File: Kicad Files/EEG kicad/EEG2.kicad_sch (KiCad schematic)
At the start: 273 parts, among them J1 Conn_02x20_Top_Bottom, J2 Conn_01x05_Pin, U1 INA823, U10 LF356M, U11 LF356M, U12 LF356M, U13 LF356M, U14 LF356M, U15 LF356M, U16 LF356M, U17 LF356M, U18 LF356M, U19 LF356M, U2 INA823, U20 LF356M, U21 LF356M, U22 LF356M, U23 LF356M, U24 LF356M, U25 LF356M, U26 AD5293, U27 AD5293, U28 AD5293, U29 AD5293, U3 INA823, U30 AD5293, U31 Teensy4.1, U32 AD5293, U33 AD5293, U34 AD5293, U35 AD5293, U36 AD5293, U37 LF356M, U38 LF356M, U39 LF356M, U4 INA823, U40 LF356M, U41 LF356M, U42 LF356M, U43 LF356M, U44 LF356M, U45 LF356M, U46 LF356M, U47 LF356M, U48 LF356M, U49 LF356M, U5 INA823, U50 LF356M, U51 LF356M, U52 LF356M, U53 LF356M, U54 LF356M, U55 LF356M, U56 LF356M, U57 INA823, U58 INA823, U59 INA823, U6 LF356M, U60 INA823, U61 INA823, U7 LF356M, U8 LF356M, U9 LF356M

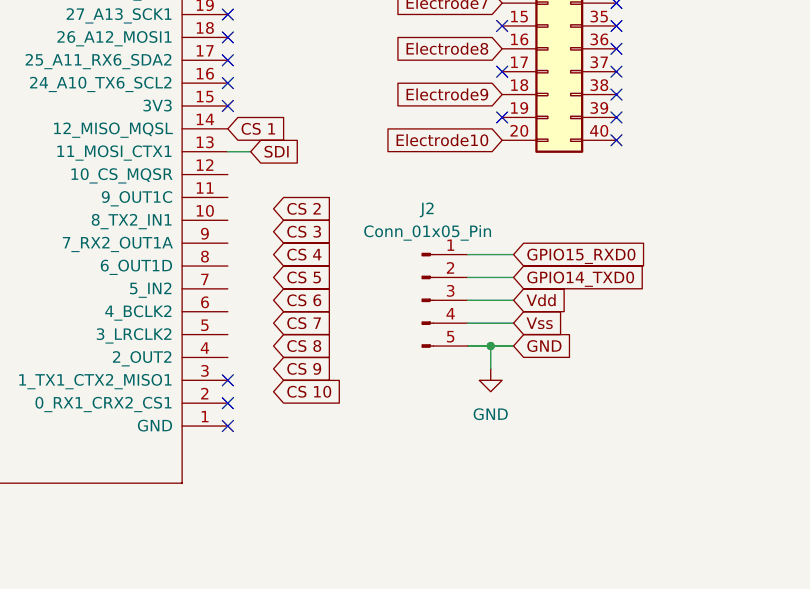
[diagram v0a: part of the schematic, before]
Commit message: AR & EEG corrected
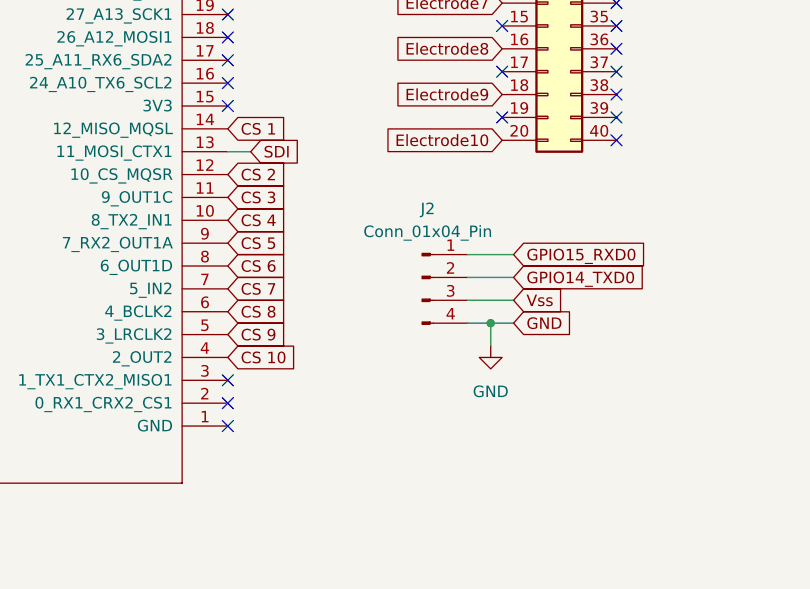
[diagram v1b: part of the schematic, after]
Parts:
- removed J2: Conn_01x05_Pin, Connector_PinHeader_1.27mm:PinHeader_1x05_P1.27mm_Vertical, symbol Connector:Conn_01x05_Pin
- added J2: Conn_01x04_Pin, Connector_PinHeader_1.27mm:PinHeader_1x04_P1.27mm_Vertical, symbol Connector:Conn_01x04_Pin
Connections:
- net CS 10: now also U31.4 (2_OUT2)
- net CS 2: now also U31.12 (10_CS_MQSR)
- net CS 3: now also U31.11 (9_OUT1C)
- net CS 4: now also U31.10 (8_TX2_IN1)
- net CS 5: now also U31.9 (7_RX2_OUT1A)
- net CS 6: now also U31.8 (6_OUT1D)
- net CS 7: now also U31.7 (5_IN2)
- net CS 8: now also U31.6 (4_BCLK2)
- net CS 9: now also U31.5 (3_LRCLK2)
- net GND: now also J2.4 (Pin_4)
- net GPIO14_TXD0: now also J2.2 (Pin_2)
- net GPIO15_RXD0: now also J2.1 (Pin_1)
- net Vss: now also J2.3 (Pin_3)
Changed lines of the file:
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@@
 	)
 	(junction
-		(at 321.31 92.71)
+		(at 321.31 90.17)
 		(diameter 0)
 		(color 0 0 0 0)
@@
 	(wire
 		(pts
-			(xy 321.31 92.71) (xy 321.31 95.25)
+			(xy 321.31 90.17) (xy 321.31 92.71)
 		)
 		(stroke
@@
 	(wire
 		(pts
-			(xy 318.77 87.63) (xy 323.85 87.63)
-		)
-		(stroke
-			(width 0)
-			(type default)
-		)
-	)
-	(wire
-		(pts
 			(xy 219.71 360.68) (xy 222.25 360.68)
 		)
@@
 	(wire
 		(pts
-			(xy 318.77 92.71) (xy 321.31 92.71)
-		)
-		(stroke
-			(width 0)
-			(type default)
-		)
-	)
-	(wire
-		(pts
-			(xy 318.77 90.17) (xy 323.85 90.17)
+			(xy 318.77 90.17) (xy 321.31 90.17)
 		)
 		(stroke
@@
 	(wire
 		(pts
+			(xy 318.77 87.63) (xy 323.85 87.63)
+		)
+		(stroke
+			(width 0)
+			(type default)
+		)
+	)
+	(wire
+		(pts
 			(xy 74.93 233.68) (xy 77.47 233.68)
 		)
@@
 	(wire
 		(pts
-			(xy 321.31 92.71) (xy 323.85 92.71)
+			(xy 321.31 90.17) (xy 323.85 90.17)
 		)
 		(stroke
@@
 	(global_label "CS 10"
 		(shape input)
-		(at 297.18 97.79 0)
+		(at 292.1 93.98 0)
 		(fields_autoplaced yes)
 		(effects
@@
 		)
 		(property "Intersheetrefs" "${INTERSHEET_REFS}"
-			(at 306.0313 97.79 0)
+			(at 300.9513 93.98 0)
 			(effects
 				(font
@@
 	(global_label "CS 9"
 		(shape input)
-		(at 297.18 95.25 0)
+		(at 292.1 91.44 0)
 		(fields_autoplaced yes)
 		(effects
@@
 		)
 		(property "Intersheetrefs" "${INTERSHEET_REFS}"
-			(at 304.8218 95.25 0)
+			(at 299.7418 91.44 0)
 			(effects
 				(font
@@
 	(global_label "GND"
 		(shape input)
-		(at 323.85 92.71 0)
+		(at 323.85 90.17 0)
 		(fields_autoplaced yes)
 		(effects
@@
 		)
 		(property "Intersheetrefs" "${INTERSHEET_REFS}"
-			(at 330.7057 92.71 0)
+			(at 330.7057 90.17 0)
 			(effects
 				(font
@@
 	(global_label "CS 4"
 		(shape input)
-		(at 297.18 82.55 0)
+		(at 292.1 78.74 0)
 		(fields_autoplaced yes)
 		(effects
@@
 		)
 		(property "Intersheetrefs" "${INTERSHEET_REFS}"
-			(at 304.8218 82.55 0)
+			(at 299.7418 78.74 0)
 			(effects
 				(font
@@
 		)
 	)
-	(global_label "Vdd"
-		(shape input)
-		(at 323.85 87.63 0)
-		(fields_autoplaced yes)
-		(effects
-			(font
-				(size 1.27 1.27)
-			)
-			(justify left)
-		)
-		(property "Intersheetrefs" "${INTERSHEET_REFS}"
-			(at 330.2218 87.63 0)
-			(effects
-				(font
-					(size 1.27 1.27)
-				)
-				(justify left)
-				(hide yes)
-			)
-		)
-	)
 	(global_label "CS 1"
 		(shape input)
@@
 	(global_label "CS 2"
 		(shape input)
-		(at 297.18 77.47 0)
+		(at 292.1 73.66 0)
 		(fields_autoplaced yes)
 		(effects
@@
 		)
 		(property "Intersheetrefs" "${INTERSHEET_REFS}"
-			(at 304.8218 77.47 0)
+			(at 299.7418 73.66 0)
 			(effects
 				(font
@@
 	(global_label "CS 5"
 		(shape input)
-		(at 297.18 85.09 0)
+		(at 292.1 81.28 0)
 		(fields_autoplaced yes)
 		(effects
@@
 		)
 		(property "Intersheetrefs" "${INTERSHEET_REFS}"
-			(at 304.8218 85.09 0)
+			(at 299.7418 81.28 0)
 			(effects
 				(font
@@
 	(global_label "CS 3"
 		(shape input)
-		(at 297.18 80.01 0)
+		(at 292.1 76.2 0)
 		(fields_autoplaced yes)
 		(effects
@@
 		)
 		(property "Intersheetrefs" "${INTERSHEET_REFS}"
-			(at 304.8218 80.01 0)
+			(at 299.7418 76.2 0)
 			(effects
 				(font
@@
 	(global_label "CS 6"
 		(shape input)
-		(at 297.18 87.63 0)
+		(at 292.1 83.82 0)
 		(fields_autoplaced yes)
 		(effects
@@
 		)
 		(property "Intersheetrefs" "${INTERSHEET_REFS}"
-			(at 304.8218 87.63 0)
+			(at 299.7418 83.82 0)
 			(effects
 				(font
@@
 	(global_label "CS 7"
 		(shape input)
-		(at 297.18 90.17 0)
+		(at 292.1 86.36 0)
 		(fields_autoplaced yes)
 		(effects
@@
 		)
 		(property "Intersheetrefs" "${INTERSHEET_REFS}"
-			(at 304.8218 90.17 0)
+			(at 299.7418 86.36 0)
 			(effects
 				(font
@@
 	(global_label "CS 8"
 		(shape input)
-		(at 297.18 92.71 0)
+		(at 292.1 88.9 0)
 		(fields_autoplaced yes)
 		(effects
@@
 		)
 		(property "Intersheetrefs" "${INTERSHEET_REFS}"
-			(at 304.8218 92.71 0)
+			(at 299.7418 88.9 0)
 			(effects
 				(font
@@
 	(global_label "Vss"
 		(shape input)
-		(at 323.85 90.17 0)
+		(at 323.85 87.63 0)
 		(fields_autoplaced yes)
 		(effects
@@
 		)
 		(property "Intersheetrefs" "${INTERSHEET_REFS}"
-			(at 329.98 90.17 0)
+			(at 329.98 87.63 0)
 			(effects
 				(font
@@
 	(symbol
 		(lib_id "power:GND")
-		(at 321.31 95.25 0)
+		(at 321.31 92.71 0)
 		(unit 1)
 		(exclude_from_sim no)
@@
 		(fields_autoplaced yes)
 		(property "Reference" "#PWR01"
-			(at 321.31 101.6 0)
+			(at 321.31 99.06 0)
 			(effects
 				(font
@@
 		)
 		(property "Value" "GND"
-			(at 321.31 100.33 0)
+			(at 321.31 97.79 0)
 			(effects
 				(font
@@
 		)
 		(property "Footprint" ""
-			(at 321.31 95.25 0)
+			(at 321.31 92.71 0)
 			(effects
 				(font
@@
 		)
 		(property "Datasheet" ""
-			(at 321.31 95.25 0)
+			(at 321.31 92.71 0)
 			(effects
 				(font
@@
 		)
 		(property "Description" "Power symbol creates a global label with name \"GND\" , ground"
-			(at 321.31 95.25 0)
+			(at 321.31 92.71 0)
 			(effects
 				(font
@@
 	)
 	(symbol
-		(lib_id "Connector:Conn_01x05_Pin")
-		(at 313.69 87.63 0)
-		(unit 1)
-		(exclude_from_sim no)
-		(in_bom yes)
-		(on_board yes)
-		(dnp no)
-		(fields_autoplaced yes)
-		(property "Reference" "J2"
-			(at 314.325 77.47 0)
-			(effects
-				(font
-					(size 1.27 1.27)
-				)
-			)
-		)
-		(property "Value" "Conn_01x05_Pin"
-			(at 314.325 80.01 0)
-			(effects
-				(font
-					(size 1.27 1.27)
-				)
-			)
-		)
-		(property "Footprint" "Connector_PinHeader_1.27mm:PinHeader_1x05_P1.27mm_Vertical"
-			(at 313.69 87.63 0)
-			(effects
-				(font
-					(size 1.27 1.27)
-				)
-				(hide yes)
-			)
-		)
-		(property "Datasheet" "~"
-			(at 313.69 87.63 0)
-			(effects
-				(font
-					(size 1.27 1.27)
-				)
-				(hide yes)
-			)
-		)
-		(property "Description" "Generic connector, single row, 01x05, script generated"
-			(at 313.69 87.63 0)
-			(effects
-				(font
-					(size 1.27 1.27)
-				)
-				(hide yes)
-			)
-		)
-		(pin "5"
-		)
-		(pin "4"
-		)
-		(pin "1"
-		)
-		(pin "2"
-		)
-		(pin "3"
-		)
-		(instances
-			(project ""
-				(path "/7738e0e1-eda6-4030-aedd-c518b834bf8b"
-					(reference "J2")
-					(unit 1)
-				)
-			)
-		)
-	)
-	(symbol
 		(lib_id "Amplifier_Instrumentation:INA333xxDGK")
 		(at 82.55 129.54 0)
@@
 					(unit 1)
 				)
+			)
+		)
+	)
+	(symbol
+		(lib_id "Connector:Conn_01x04_Pin")
+		(at 313.69 85.09 0)
+		(unit 1)
+		(exclude_from_sim no)
+		(in_bom yes)
+		(on_board yes)
+		(dnp no)
+		(fields_autoplaced yes)
+		(property "Reference" "J2"
+			(at 314.325 77.47 0)
+			(effects
+				(font
+					(size 1.27 1.27)
+				)
+			)
+		)
+		(property "Value" "Conn_01x04_Pin"
+			(at 314.325 80.01 0)
+			(effects
+				(font
+					(size 1.27 1.27)
+				)
+			)
+		)
+		(property "Footprint" "Connector_PinHeader_1.27mm:PinHeader_1x04_P1.27mm_Vertical"
+			(at 313.69 85.09 0)
+			(effects
+				(font
+					(size 1.27 1.27)
+				)
+				(hide yes)
+			)
+		)
+		(property "Datasheet" "~"
+			(at 313.69 85.09 0)
+			(effects
+				(font
+					(size 1.27 1.27)
+				)
+				(hide yes)
+			)
+		)
+		(property "Description" "Generic connector, single row, 01x04, script generated"
+			(at 313.69 85.09 0)
+			(effects
+				(font
+					(size 1.27 1.27)
+				)
+				(hide yes)
+			)
+		)
+		(pin "2"
+		)
+		(pin "4"
+		)
+		(pin "1"
+		)
+		(pin "3"
+		)
+		(instances
+			(project ""
+				(path "/7738e0e1-eda6-4030-aedd-c518b834bf8b"
+					(reference "J2")
+					(unit 1)
+				)
